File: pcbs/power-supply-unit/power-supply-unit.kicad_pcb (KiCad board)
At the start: 2 copper layers, 37.5 x 86 mm, 24 parts, among them J1 BMS_OUTPUT, J2 PWR_CONN_RASPI, J3 PWR_CONN_CTRL, U1 LM2576S-ADJ, U2 LM2576S-ADJ, U3 AMS1117-3.3

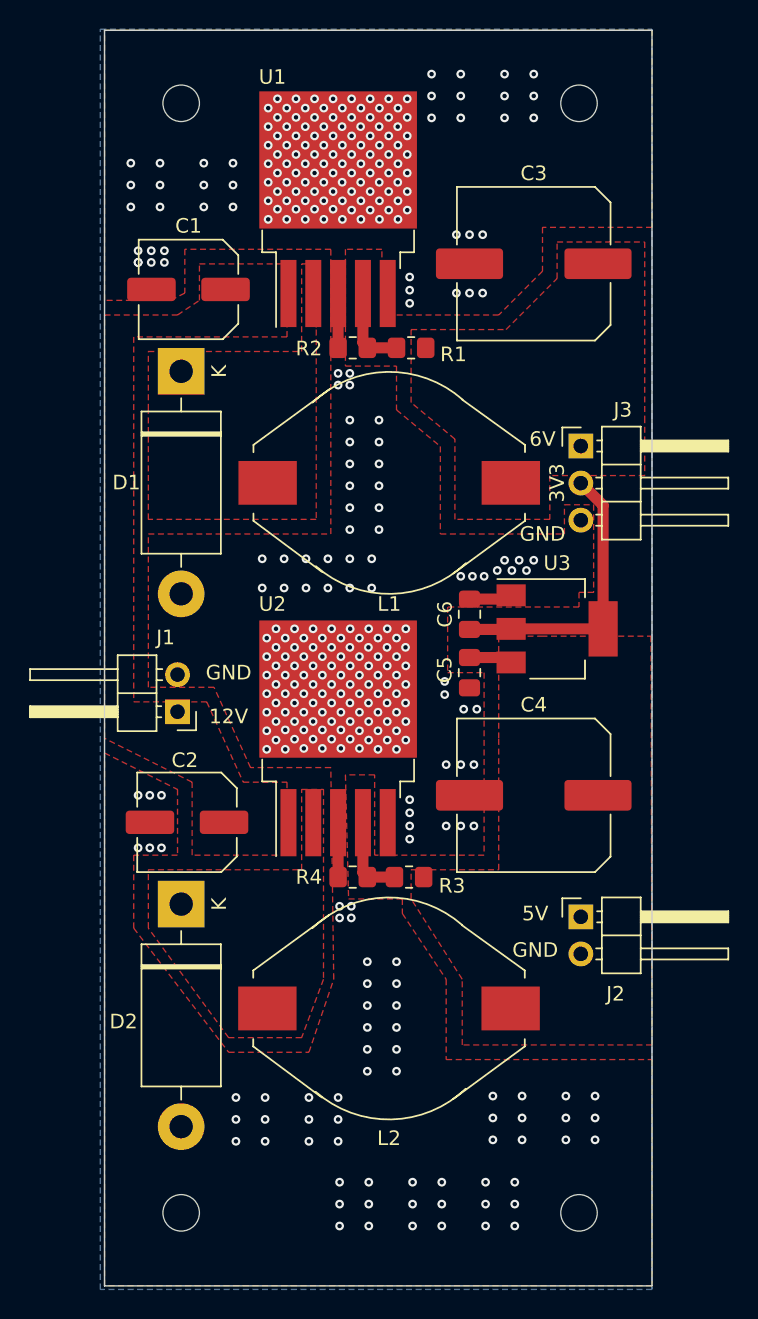
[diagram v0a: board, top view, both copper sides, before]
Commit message: Fix mounting hole position inaccuracy with pwr-supply
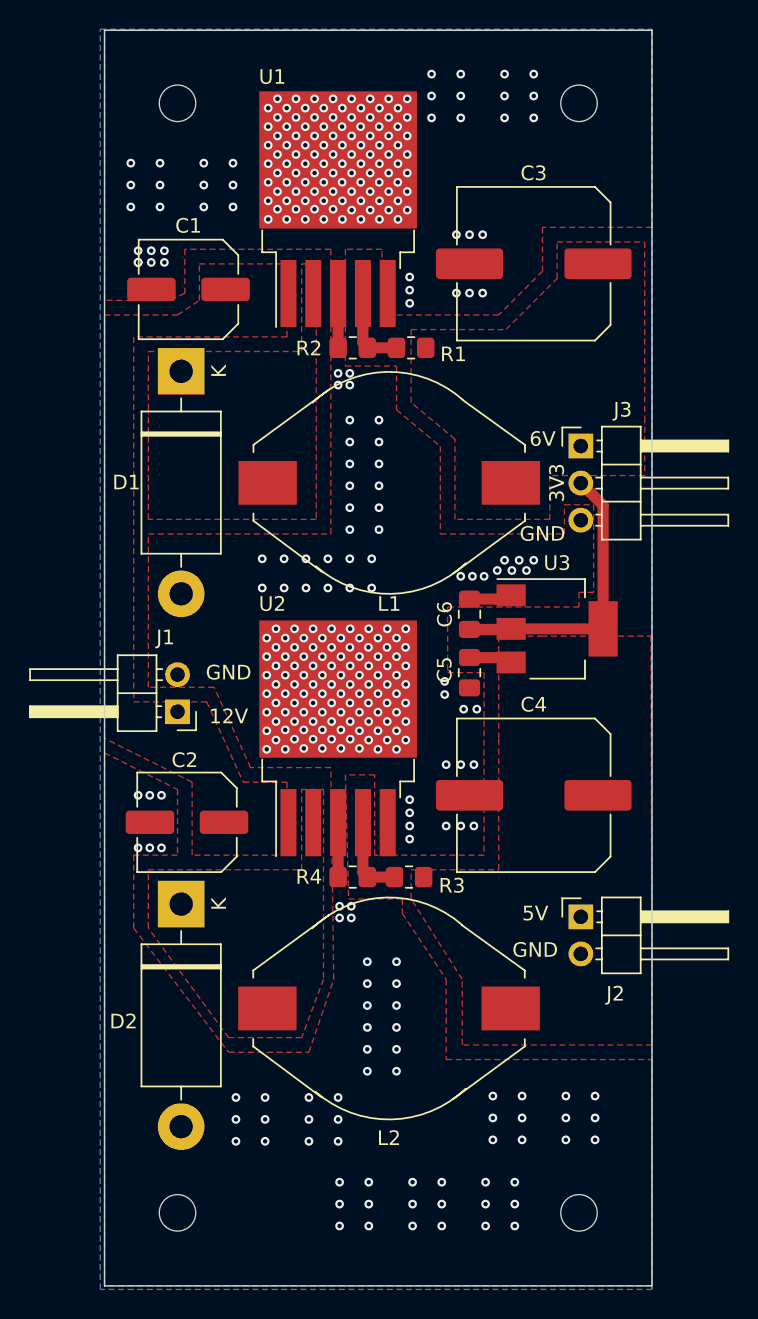
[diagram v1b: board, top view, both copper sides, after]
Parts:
- moved REF02 0.25 mm to (110.0, 115.0)
- moved REF03 0.25 mm to (110.0, 39.0)
